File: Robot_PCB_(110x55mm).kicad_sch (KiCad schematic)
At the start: 19 parts, among them U1 L293, U2 SW_DPDT_XLX, U3 AMS1117-5.0, U5 MFRC522 37.5x25mm

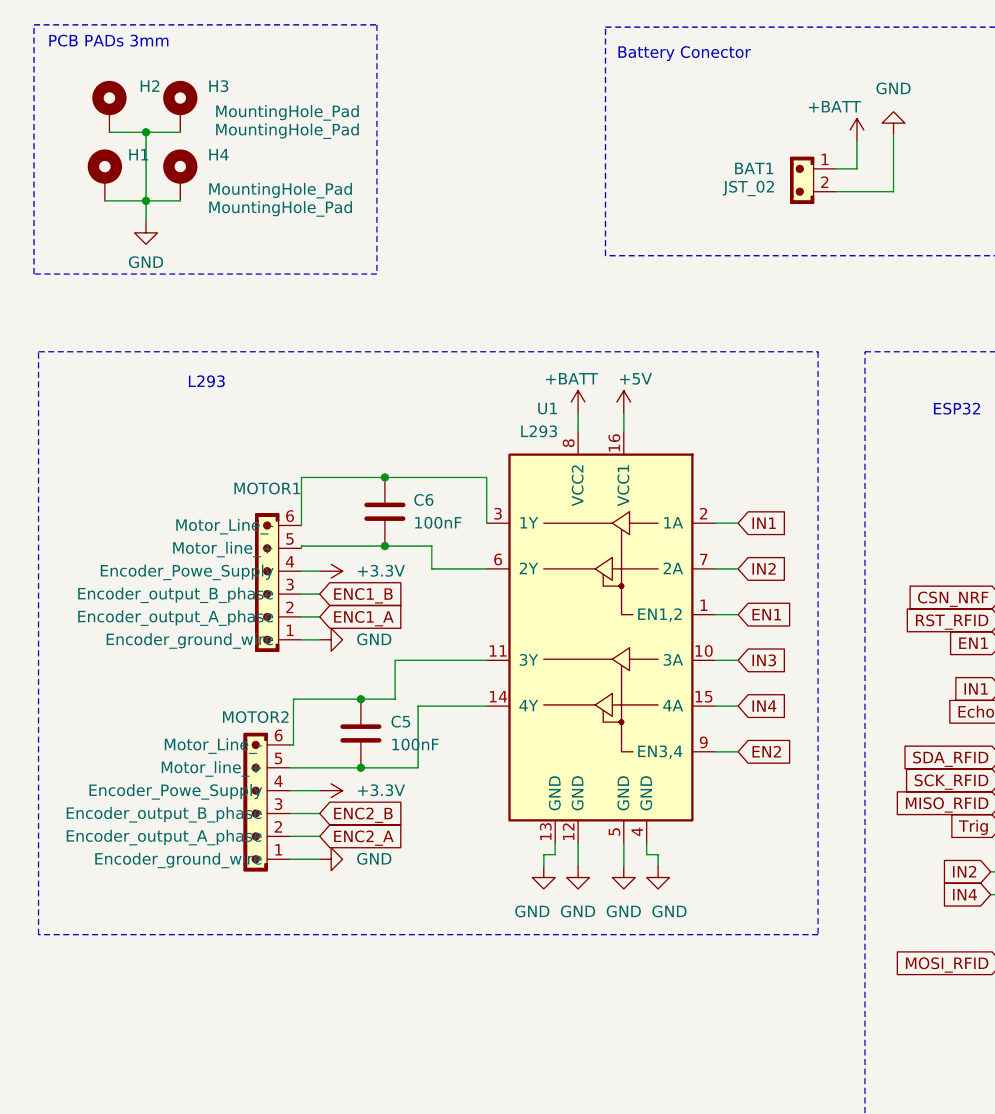
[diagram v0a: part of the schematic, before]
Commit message: update
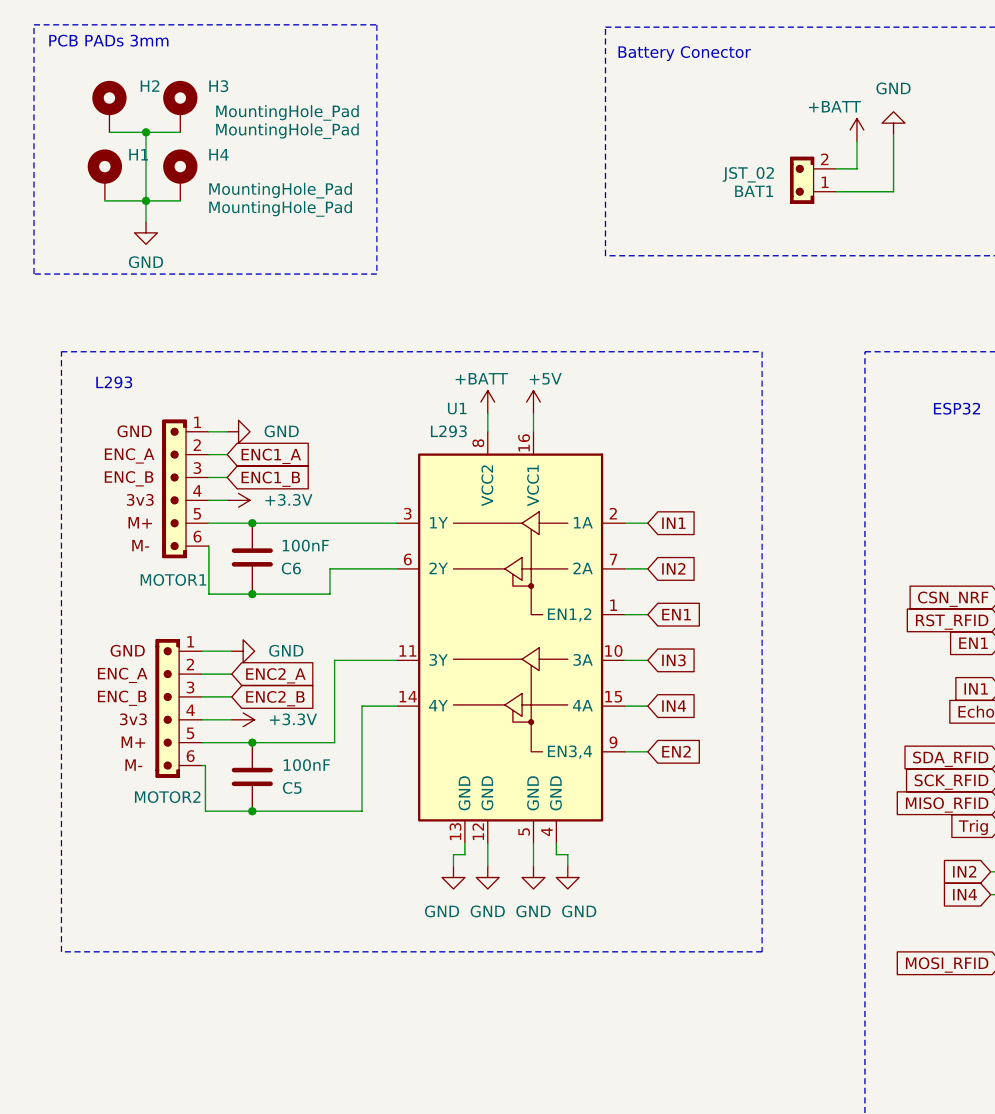
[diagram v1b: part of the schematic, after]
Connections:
- net +BATT: now also BAT1.2; no longer BAT1.1
- net GND: now also BAT1.1; no longer BAT1.2
- net at C5.2, MOTOR2.5: now also U1.11 (3Y); no longer U1.14 (4Y)
- net at C5.1, MOTOR2.6: now also U1.14 (4Y); no longer U1.11 (3Y)
- net at C6.2, MOTOR1.5: now also U1.3 (1Y); no longer U1.6 (2Y)
- net at C6.1, MOTOR1.6: now also U1.6 (2Y); no longer U1.3 (1Y)
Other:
- moved on the sheet: BAT1, C5, C6, MOTOR1, MOTOR2, U1

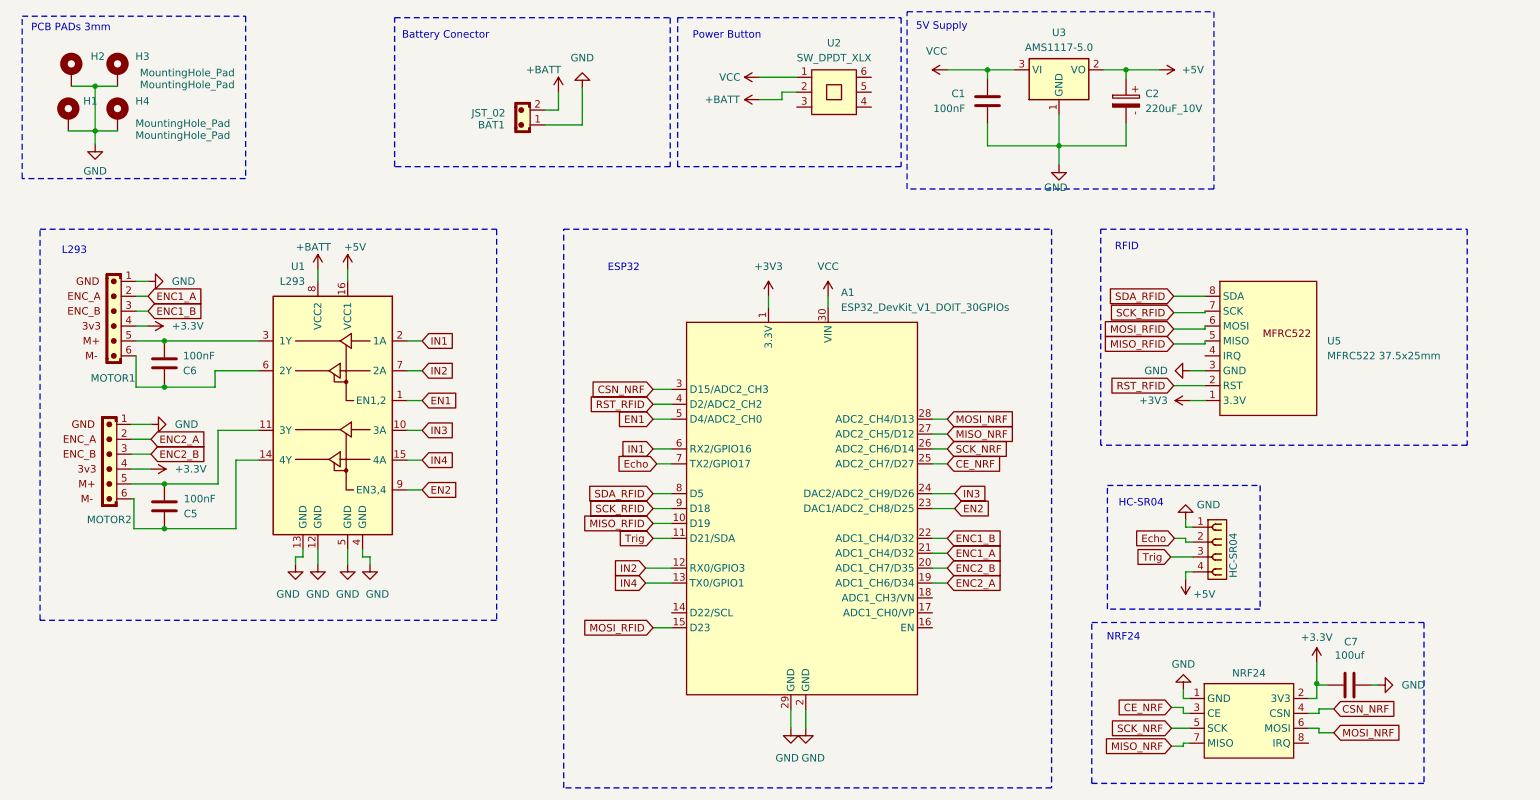
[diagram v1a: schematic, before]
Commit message: Update
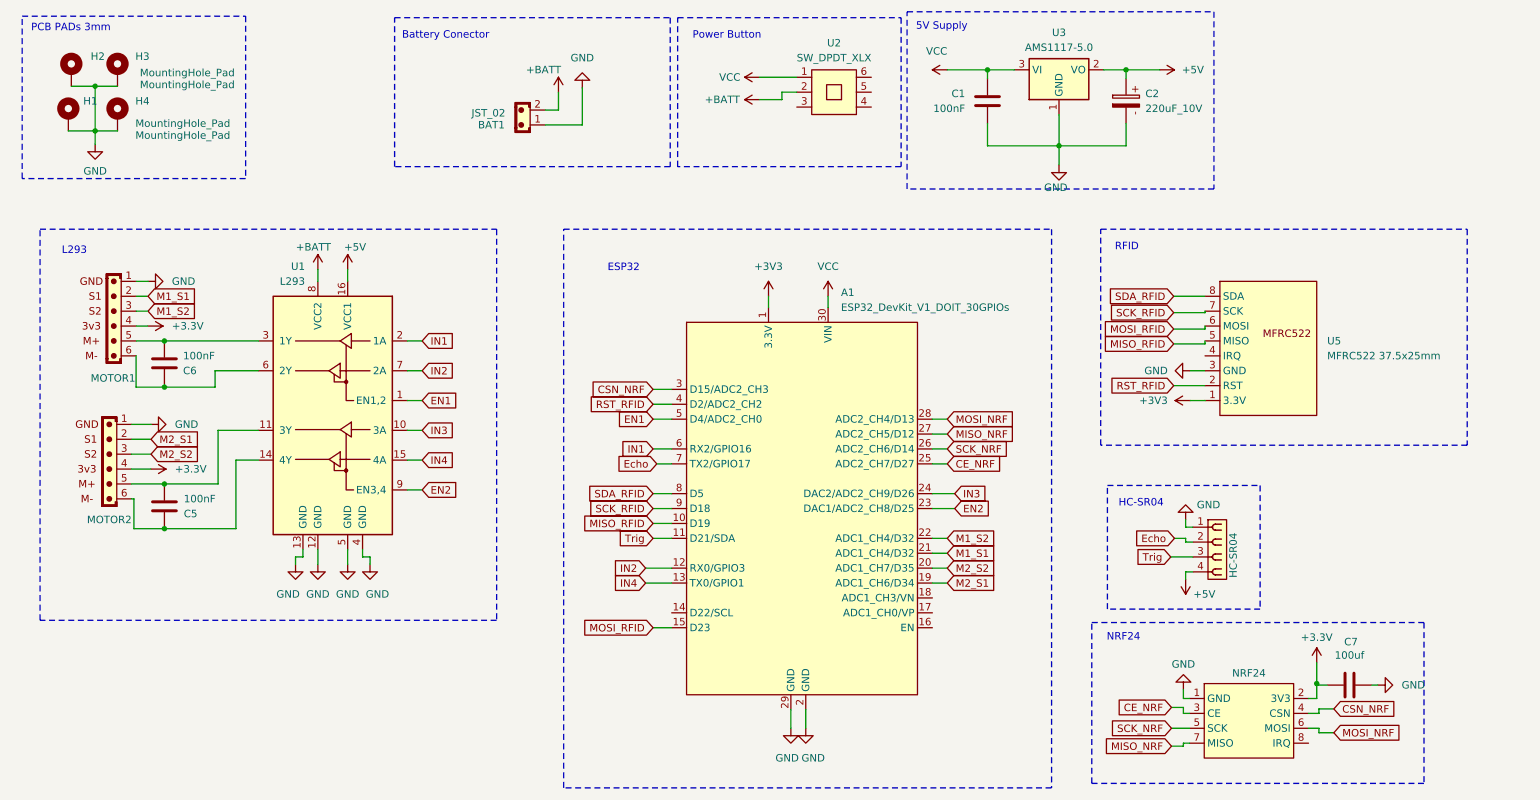
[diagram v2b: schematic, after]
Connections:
- net ENC1_A renamed M1_S1
- net ENC1_B renamed M1_S2
- net ENC2_A renamed M2_S1
- net ENC2_B renamed M2_S2
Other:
- moved on the sheet: MOTOR1, MOTOR2
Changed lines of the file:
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@@
     (effects (font (size 1.27 1.27)) (justify right bottom))
   )
-  (global_label "ENC1_B" (shape input) (at 36.449 73.66 0) (fields_autoplaced)
-    (effects (font (size 1.27 1.27)) (justify left))
-    (property "Intersheetrefs" "${INTERSHEET_REFS}" (at 46.6308 73.66 0)
+  (global_label "M1_S2" (shape input) (at 36.449 73.66 0) (fields_autoplaced)
+    (effects (font (size 1.27 1.27)) (justify left))
+    (property "Intersheetrefs" "${INTERSHEET_REFS}" (at 45.4817 73.66 0)
       (effects (font (size 1.27 1.27)) (justify left) hide)
     )
@@
     )
   )
-  (global_label "ENC2_A" (shape input) (at 36.957 95.504 0) (fields_autoplaced)
-    (effects (font (size 1.27 1.27)) (justify left))
-    (property "Intersheetrefs" "${INTERSHEET_REFS}" (at 46.9574 95.504 0)
+  (global_label "M2_S1" (shape input) (at 36.957 95.504 0) (fields_autoplaced)
+    (effects (font (size 1.27 1.27)) (justify left))
+    (property "Intersheetrefs" "${INTERSHEET_REFS}" (at 45.9897 95.504 0)
       (effects (font (size 1.27 1.27)) (justify left) hide)
     )
@@
     )
   )
-  (global_label "ENC2_B" (shape input) (at 172.72 117.475 0) (fields_autoplaced)
-    (effects (font (size 1.27 1.27)) (justify left))
-    (property "Intersheetrefs" "${INTERSHEET_REFS}" (at 182.9018 117.475 0)
+  (global_label "M2_S2" (shape input) (at 172.72 117.475 0) (fields_autoplaced)
+    (effects (font (size 1.27 1.27)) (justify left))
+    (property "Intersheetrefs" "${INTERSHEET_REFS}" (at 181.7527 117.475 0)
       (effects (font (size 1.27 1.27)) (justify left) hide)
     )
@@
     )
   )
-  (global_label "ENC1_B" (shape input) (at 172.72 112.395 0) (fields_autoplaced)
-    (effects (font (size 1.27 1.27)) (justify left))
-    (property "Intersheetrefs" "${INTERSHEET_REFS}" (at 182.9018 112.395 0)
+  (global_label "M1_S2" (shape input) (at 172.72 112.395 0) (fields_autoplaced)
+    (effects (font (size 1.27 1.27)) (justify left))
+    (property "Intersheetrefs" "${INTERSHEET_REFS}" (at 181.7527 112.395 0)
       (effects (font (size 1.27 1.27)) (justify left) hide)
     )
@@
     )
   )
-  (global_label "ENC1_A" (shape input) (at 172.72 114.935 0) (fields_autoplaced)
-    (effects (font (size 1.27 1.27)) (justify left))
-    (property "Intersheetrefs" "${INTERSHEET_REFS}" (at 182.7204 114.935 0)
+  (global_label "M1_S1" (shape input) (at 172.72 114.935 0) (fields_autoplaced)
+    (effects (font (size 1.27 1.27)) (justify left))
+    (property "Intersheetrefs" "${INTERSHEET_REFS}" (at 181.7527 114.935 0)
       (effects (font (size 1.27 1.27)) (justify left) hide)
     )
@@
     )
   )
-  (global_label "ENC1_A" (shape input) (at 36.449 71.12 0) (fields_autoplaced)
-    (effects (font (size 1.27 1.27)) (justify left))
-    (property "Intersheetrefs" "${INTERSHEET_REFS}" (at 46.4494 71.12 0)
+  (global_label "M1_S1" (shape input) (at 36.449 71.12 0) (fields_autoplaced)
+    (effects (font (size 1.27 1.27)) (justify left))
+    (property "Intersheetrefs" "${INTERSHEET_REFS}" (at 45.4817 71.12 0)
       (effects (font (size 1.27 1.27)) (justify left) hide)
     )
@@
     )
   )
-  (global_label "ENC2_A" (shape input) (at 172.72 120.015 0) (fields_autoplaced)
-    (effects (font (size 1.27 1.27)) (justify left))
-    (property "Intersheetrefs" "${INTERSHEET_REFS}" (at 182.7204 120.015 0)
+  (global_label "M2_S1" (shape input) (at 172.72 120.015 0) (fields_autoplaced)
+    (effects (font (size 1.27 1.27)) (justify left))
+    (property "Intersheetrefs" "${INTERSHEET_REFS}" (at 181.7527 120.015 0)
       (effects (font (size 1.27 1.27)) (justify left) hide)
     )
@@
     )
   )
-  (global_label "ENC2_B" (shape input) (at 36.957 98.044 0) (fields_autoplaced)
-    (effects (font (size 1.27 1.27)) (justify left))
-    (property "Intersheetrefs" "${INTERSHEET_REFS}" (at 47.1388 98.044 0)
+  (global_label "M2_S2" (shape input) (at 36.957 98.044 0) (fields_autoplaced)
+    (effects (font (size 1.27 1.27)) (justify left))
+    (property "Intersheetrefs" "${INTERSHEET_REFS}" (at 45.9897 98.044 0)
       (effects (font (size 1.27 1.27)) (justify left) hide)
     )
@@
     )
   )
-  (symbol (lib_id "GERE_symbols:MOTOR ENC JST_06 (PH2.0) Horizontal") (at 36.195 90.424 180) (unit 1)
+  (symbol (lib_name "MOTOR ENC JST_06 (PH2.0) Horizontal_1") (lib_id "GERE_symbols:MOTOR ENC JST_06 (PH2.0) Horizontal") (at 36.195 90.424 180) (unit 1)
     (in_bom yes) (on_board yes) (dnp no)
     (property "Reference" "MOTOR2" (at 29.845 109.22 0)

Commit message: Update
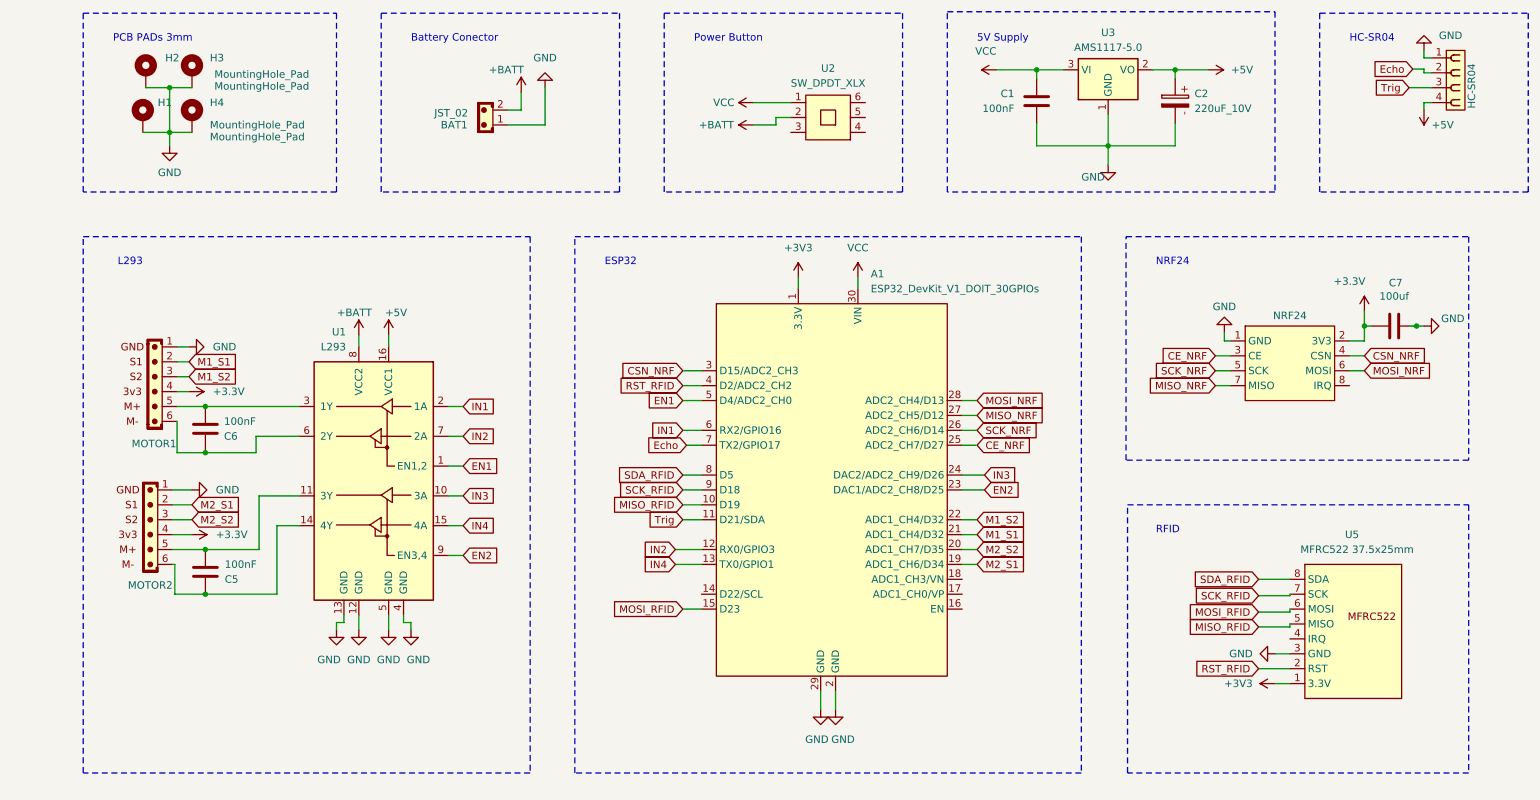
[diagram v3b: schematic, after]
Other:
- moved on the sheet: A1, BAT1, C1, C2, C5, C6, C7, H1, H2, H3, H4, HC-SR04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

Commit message: Update
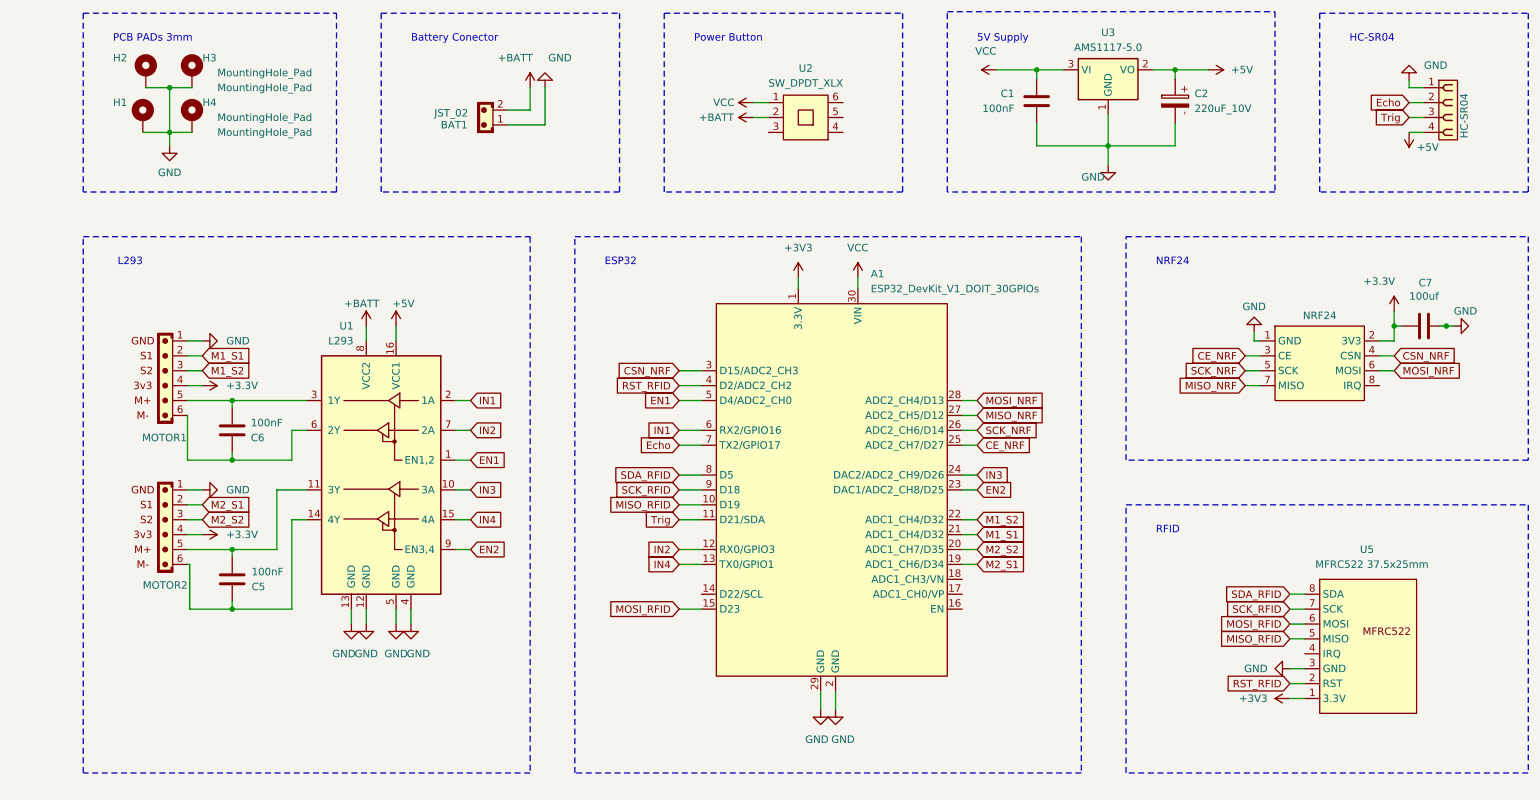
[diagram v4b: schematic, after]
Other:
- title: Robot PIBID -> Robot 2WD
- moved on the sheet: C5, C6, C7, HC-SR04, MOTOR1, MOTOR2, U1, U2, U5
